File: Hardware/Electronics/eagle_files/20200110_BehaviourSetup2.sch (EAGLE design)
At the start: 21 parts, among them Q1 IRF540, Q2 IRF540, Q3 IRF540

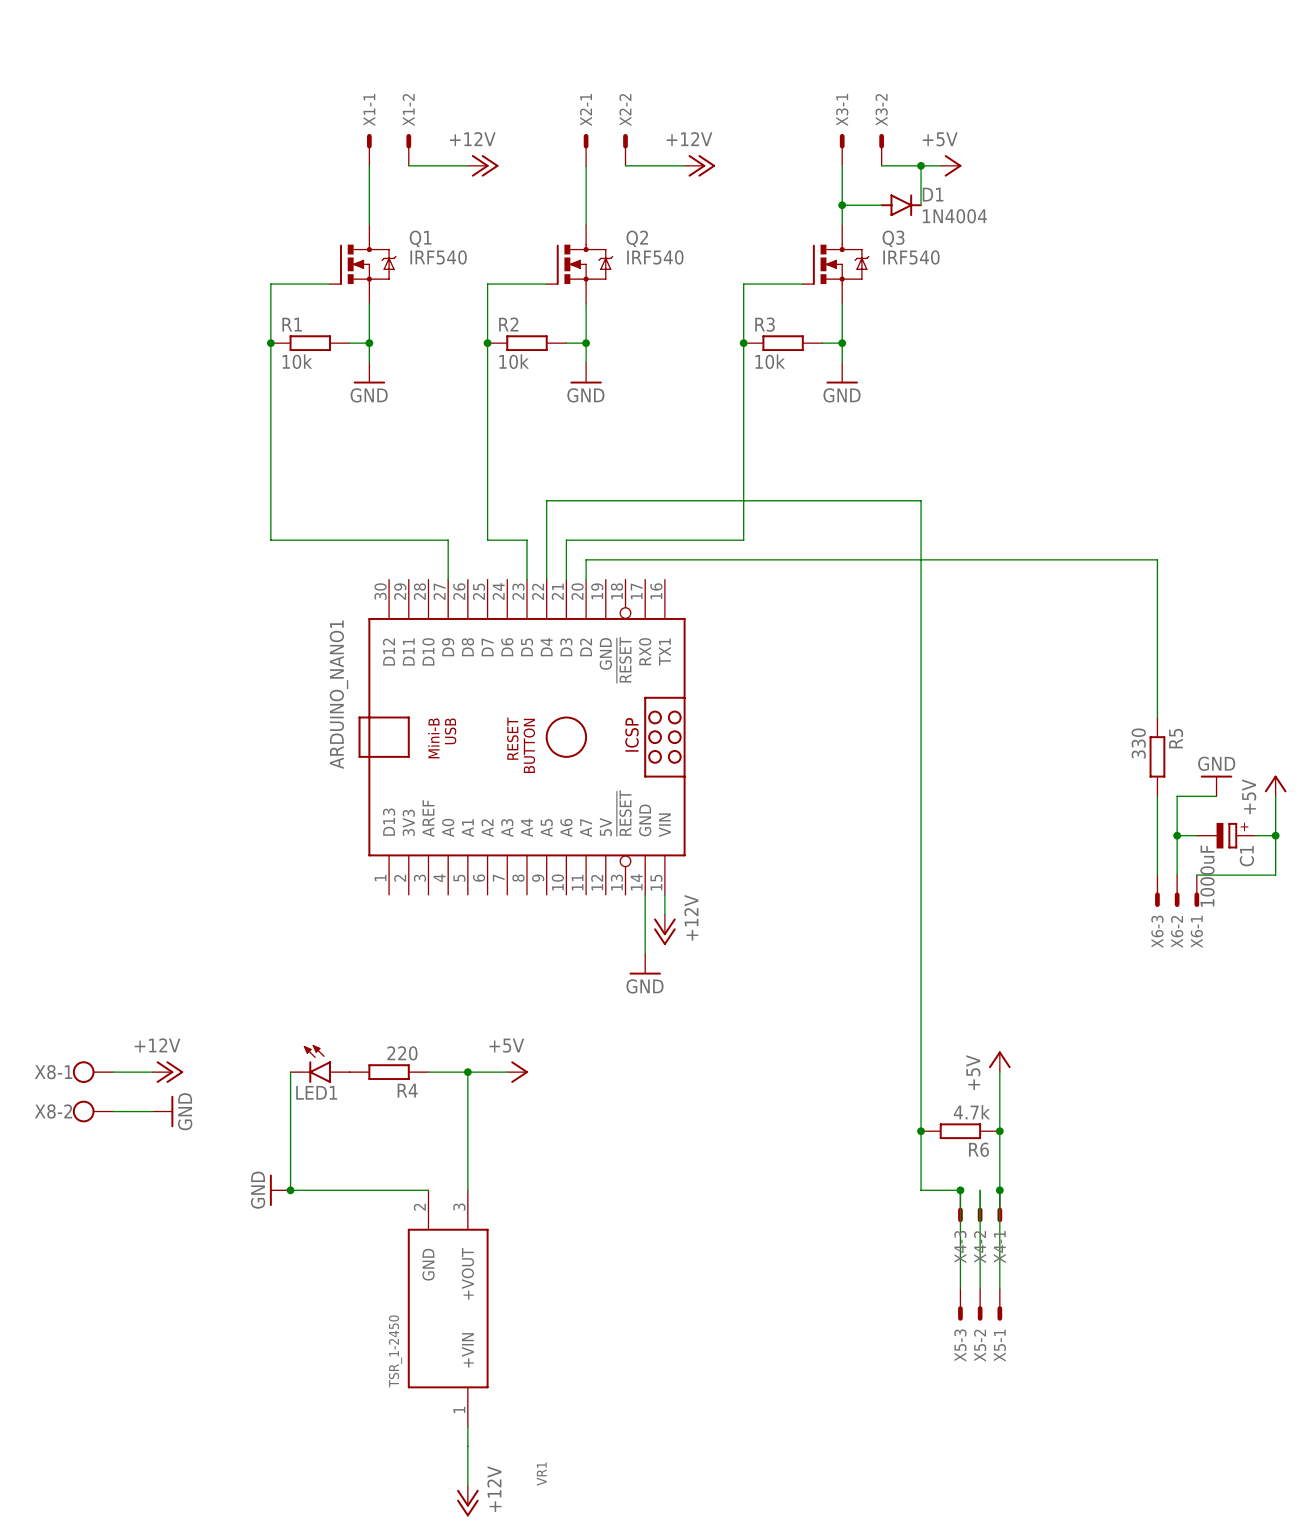
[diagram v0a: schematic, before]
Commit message: Changed circuitry, rebuilt PCB
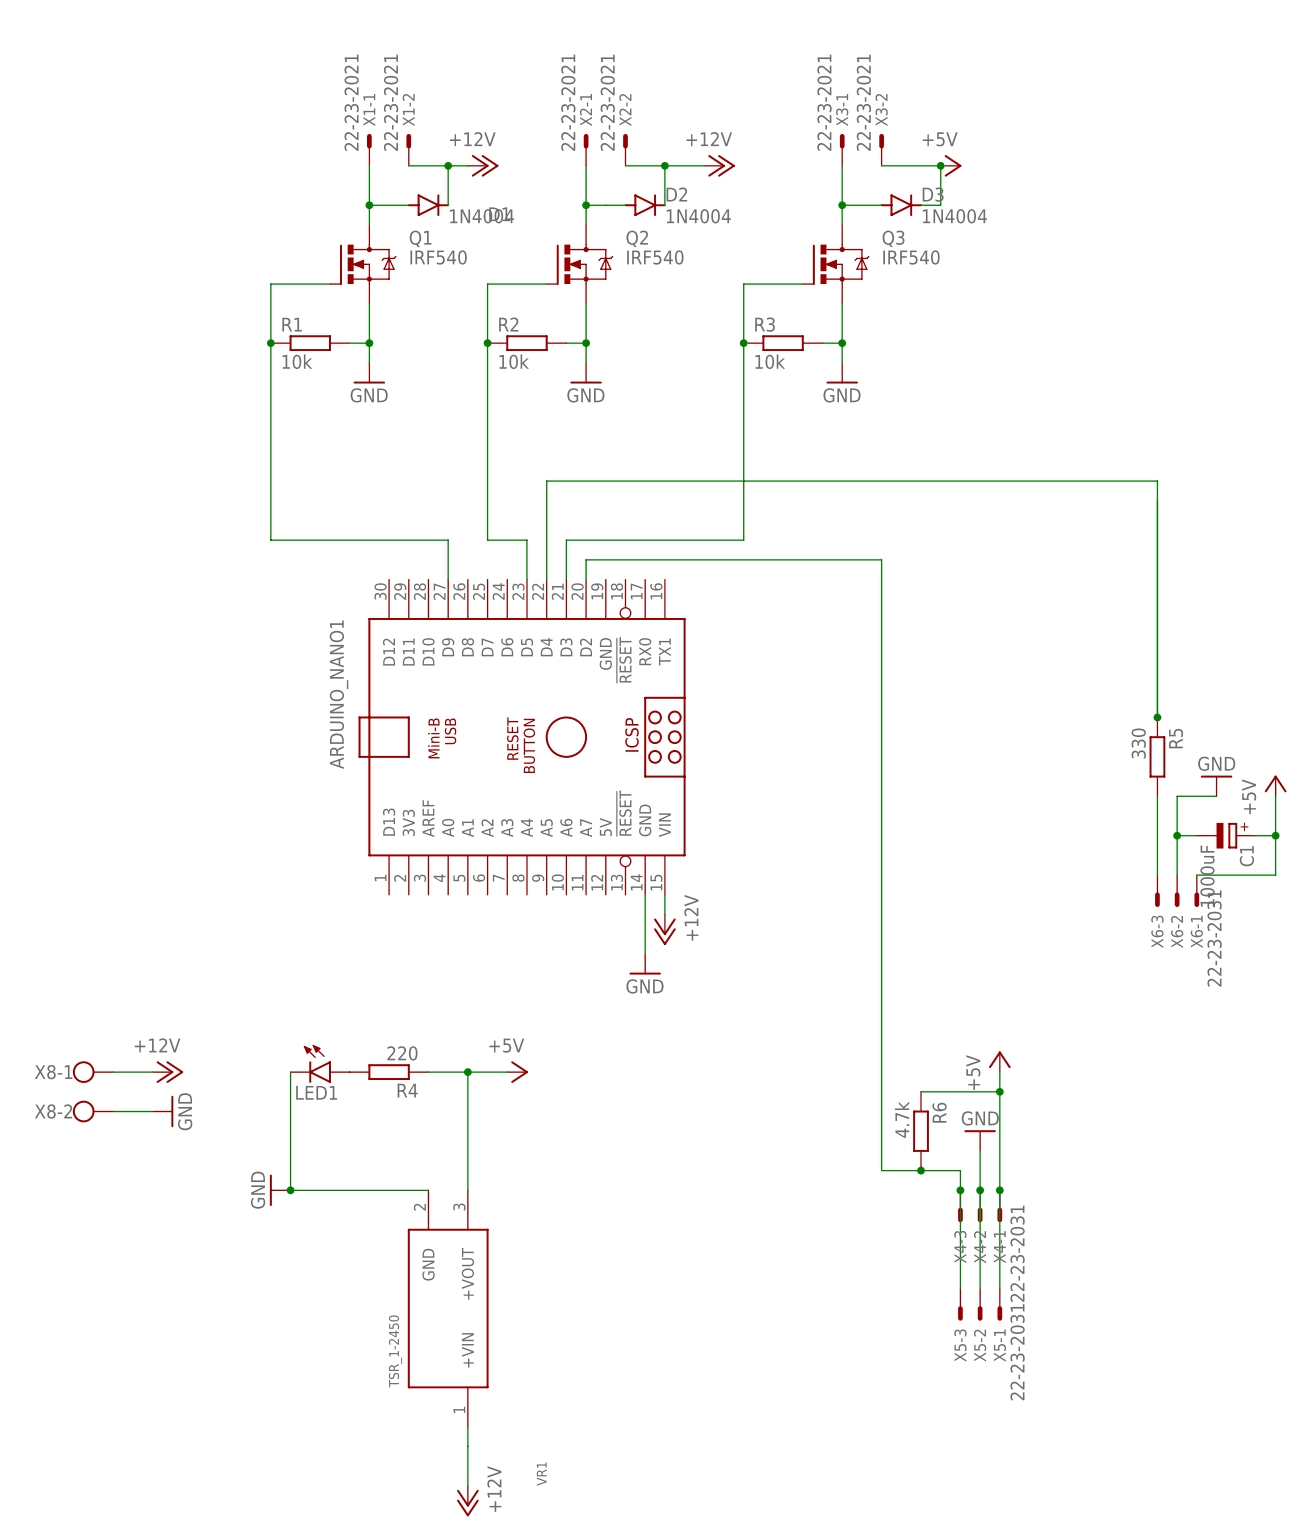
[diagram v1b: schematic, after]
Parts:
- added D2, D3: 1N4004, diode:1N4004
- C1: device rcl:CPOL-EUE3.5-10 -> rcl:CPOL-EUE5-8.5
- X1, X2, X3: value (none) -> 22-23-2021; device con-molex:KK-156-2 -> con-molex:22-23-2021
- X4, X5, X6: value (none) -> 22-23-2031; device con-molex:KK-156-3 -> con-molex:22-23-2031
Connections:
- removed net N$2: Q1.D, X1-1.S
- removed net N$8: ARDUINO_NANO1.D4, R6.2, X4-3.S, X5-3.S
- removed net N$9: X4-2.S, X5-2.S
- new net N$12: D2.A, Q2.D, X2-1.S
- new net N$13: D1.A, Q1.D, X1-1.S
- net +12V: now also D1.C, D2.C
- net +5V: now also D3.C; no longer D1.C
- net GND: now also X4-2.S, X5-2.S
- net N$10: now also ARDUINO_NANO1.D4; no longer ARDUINO_NANO1.D2
- net N$4: now also ARDUINO_NANO1.D2, R6.2, X4-3.S, X5-3.S; no longer Q2.D, X2-1.S
- net N$6: now also D3.A; no longer D1.A
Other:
- moved on the sheet: D1, R6
